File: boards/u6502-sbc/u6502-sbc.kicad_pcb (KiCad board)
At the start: 4 copper layers, 100 x 100 mm, 35 parts, among them J1 HDR_USR_PORT, J2 HDR_USR_PORT, J3 HDR_USR_PORT, J4 HDR_USR_PORT, J6 HDR_FTDI, J7 HDR_RS232, J8 KLDX-0202-BC, J9 HDR_CPU_BUS, SW1 SW_RST, SW2 SW_SPDT, U1 W65C02SxPL, U10 DS1813-5+, U2 AS7C256B-15PIN, U3 28C256, U4 W65C22SxPL, U5 W65C51NxP, U6 74HC00, U7 74HC21, U8 W65C22SxPL, U9 NCP1117IDT50T4G, X1 1MHz

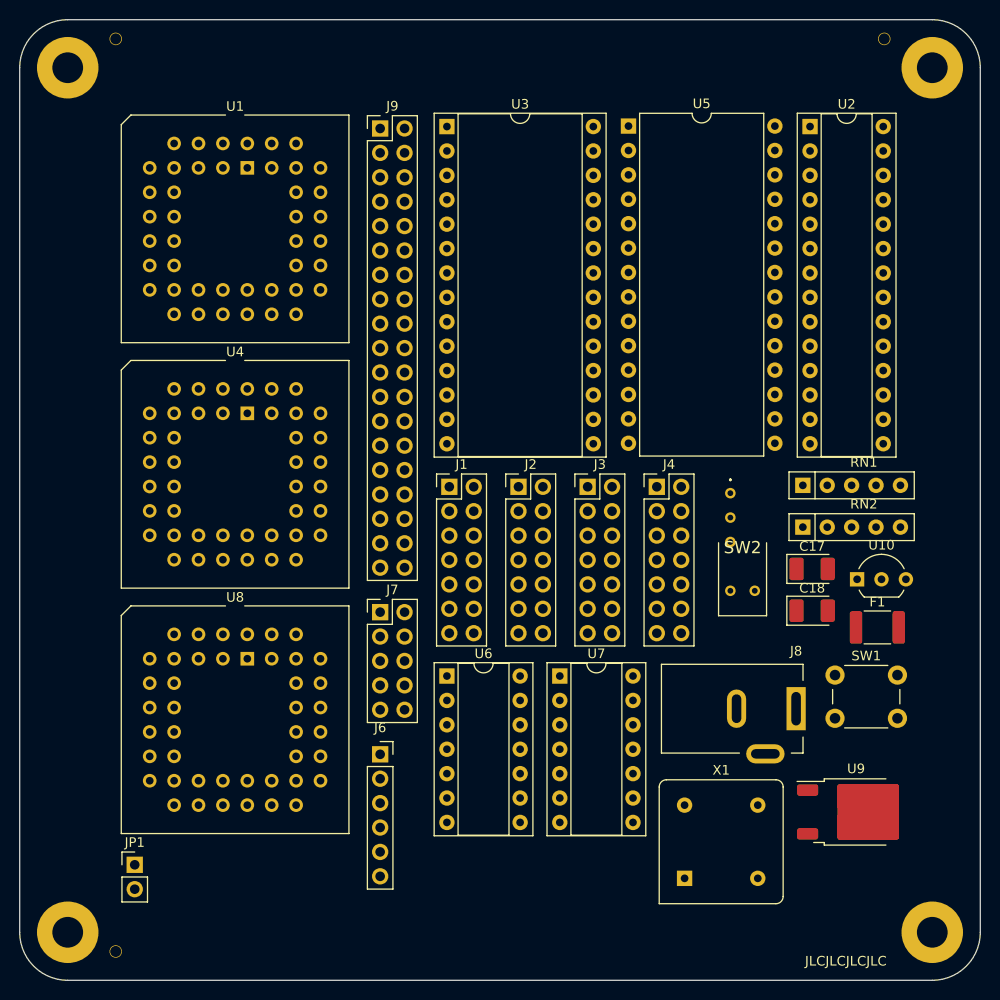
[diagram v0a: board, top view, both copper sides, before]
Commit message: Initial layout and routing wip
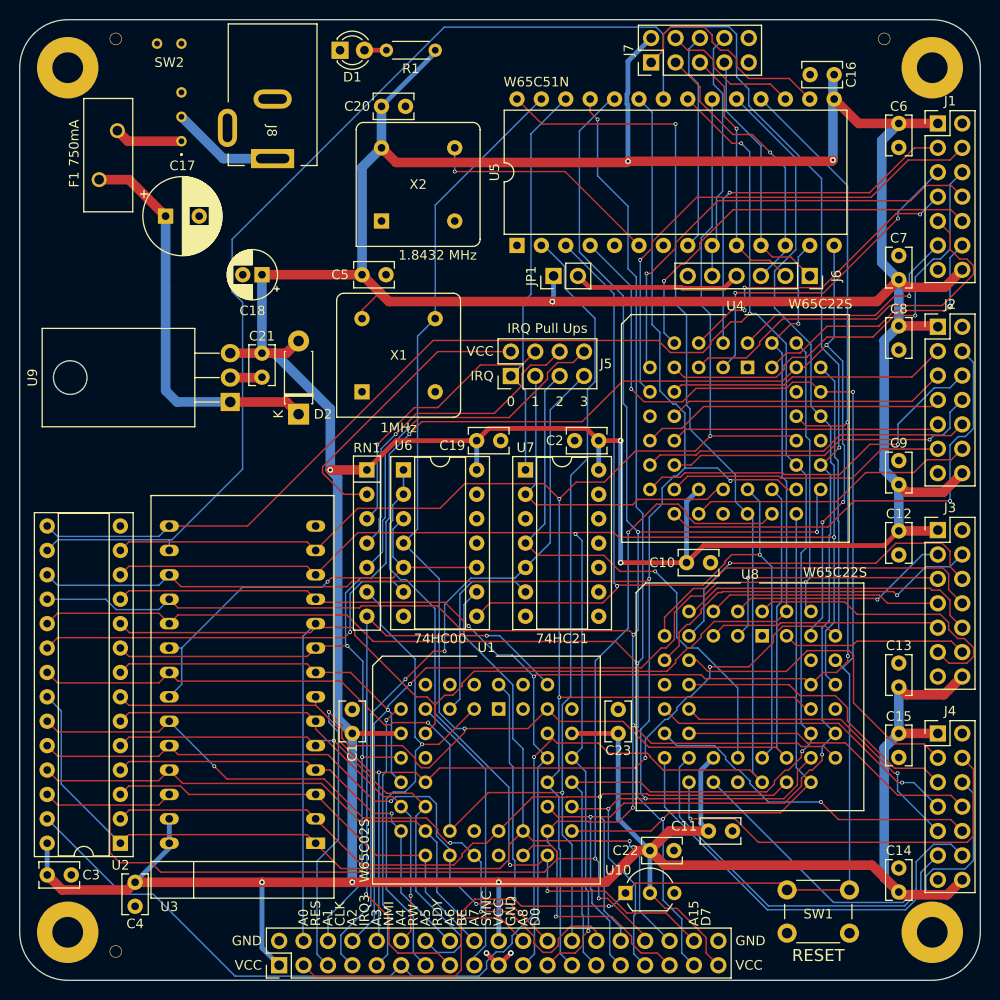
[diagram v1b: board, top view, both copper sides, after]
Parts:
- removed RN2: 3k3, Resistor_THT:R_Array_SIP5
- added C1: 100n, Capacitor_THT:C_Rect_L4.0mm_W2.5mm_P2.50mm, F.Cu at (134.6, 114.3)
- added C10: 100n, Capacitor_THT:C_Rect_L4.0mm_W2.5mm_P2.50mm, F.Cu at (169.4, 96.5)
- added C11: 100n, Capacitor_THT:C_Rect_L4.0mm_W2.5mm_P2.50mm, F.Cu at (171.7, 124.5)
- added C12: 100n, Capacitor_THT:C_Rect_L4.0mm_W2.5mm_P2.50mm, F.Cu at (191.5, 93.2)
- added C13: 100n, Capacitor_THT:C_Rect_L4.0mm_W2.5mm_P2.50mm, F.Cu at (191.5, 109.5)
- added C14: 100n, Capacitor_THT:C_Rect_L4.0mm_W2.5mm_P2.50mm, F.Cu at (191.5, 130.8)
- added C15: 100n, Capacitor_THT:C_Rect_L4.0mm_W2.5mm_P2.50mm, F.Cu at (191.5, 114.3)
- added C16: 100n, Capacitor_THT:C_Rect_L4.0mm_W2.5mm_P2.50mm, F.Cu at (184.8, 45.7)
- added C19: 100n, Capacitor_THT:C_Rect_L4.0mm_W2.5mm_P2.50mm, F.Cu at (147.6, 83.8)
- added C2: 100n, Capacitor_THT:C_Rect_L4.0mm_W2.5mm_P2.50mm, F.Cu at (160.3, 83.8)
- added C20: 100n, Capacitor_THT:C_Rect_L4.0mm_W2.5mm_P2.50mm, F.Cu at (140.2, 49.0)
- added C21: 100n, Capacitor_THT:C_Rect_L4.0mm_W2.5mm_P2.50mm, F.Cu at (125.2, 74.7)
- added C22: 100n, Capacitor_THT:C_Rect_L4.0mm_W2.5mm_P2.50mm, F.Cu at (165.6, 126.5)
- added C23: 100n, Capacitor_THT:C_Rect_L4.0mm_W2.5mm_P2.50mm, F.Cu at (162.3, 114.3)
- added C3: 100n, Capacitor_THT:C_Rect_L4.0mm_W2.5mm_P2.50mm, F.Cu at (102.9, 129.0)
- added C4: 100n, Capacitor_THT:C_Rect_L4.0mm_W2.5mm_P2.50mm, F.Cu at (112.0, 129.8)
- added C5: 100n, Capacitor_THT:C_Rect_L4.0mm_W2.5mm_P2.50mm, F.Cu at (135.6, 66.5)
- added C6: 100n, Capacitor_THT:C_Rect_L4.0mm_W2.5mm_P2.50mm, F.Cu at (191.5, 50.8)
- added C7: 100n, Capacitor_THT:C_Rect_L4.0mm_W2.5mm_P2.50mm, F.Cu at (191.5, 67.1)
- added C8: 100n, Capacitor_THT:C_Rect_L4.0mm_W2.5mm_P2.50mm, F.Cu at (191.5, 71.9)
- added C9: 100n, Capacitor_THT:C_Rect_L4.0mm_W2.5mm_P2.50mm, F.Cu at (191.5, 88.4)
- added D1: LED_PWR, LED_THT:LED_D3.0mm, F.Cu at (133.3, 43.2)
- added D2: 1N5819, Diode_THT:D_DO-41_SOD81_P7.62mm_Horizontal, F.Cu at (129.0, 81.1)
- added J5: HDR_IRQ, Connector_PinHeader_2.54mm:PinHeader_2x04_P2.54mm_Vertical, F.Cu at (151.1, 77.1)
- added R1: 1k, Resistor_THT:R_Axial_DIN0204_L3.6mm_D1.6mm_P5.08mm_Horizontal, F.Cu at (143.3, 43.2)
- added X2: 1.8432 MHz, Oscillator:Oscillator_DIP-8, F.Cu at (137.7, 61.0)
- C17: footprint Capacitor_Tantalum_SMD:CP_EIA-3528-21_Kemet-B_Pad1.50x2.35mm_HandSolder -> Capacitor_THT:CP_Radial_D8.0mm_P3.50mm
- C18: value 10u -> 4u7; footprint Capacitor_Tantalum_SMD:CP_EIA-3528-21_Kemet-B_Pad1.50x2.35mm_HandSolder -> Capacitor_THT:CP_Radial_D5.0mm_P2.00mm
- F1: footprint Fuse:Fuse_1812_4532Metric_Pad1.30x3.40mm_HandSolder -> Fuse:Fuse_BelFuse_0ZRE0075FF_L11.5mm_W4.8mm
- RN1: footprint Resistor_THT:R_Array_SIP5 -> Resistor_THT:R_Array_SIP7
- SYM1: moved to B.Cu
- U3: footprint Package_DIP:DIP-28_W15.24mm_Socket -> Mouser:Aries 28-526-10
- U9: value NCP1117IDT50T4G -> L7805CV; footprint Package_TO_SOT_SMD:TO-252-2 -> Package_TO_SOT_THT:TO-220-3_Horizontal_TabDown
- moved U2 103.5 mm to (110.5, 125.7), turned to 180 degrees
- moved F1 94.5 mm to (110.2, 51.6), turned to -90 degrees
- moved locked 87.7 mm to (127.0, 138.4), turned to 90 degrees
- moved J8 79.1 mm to (126.3, 54.5), turned to -90 degrees
- moved U9 77.9 mm to (121.9, 79.8), turned to 90 degrees
- moved C17 76.7 mm to (115.2, 60.5)
- moved JP1 75.2 mm to (155.6, 66.7), turned to 90 degrees
- moved SW2 67.9 mm to (116.8, 52.6), turned to 180 degrees
- moved C18 67.1 mm to (125.2, 66.5), turned to 180 degrees
- moved J6 66.9 mm to (182.2, 66.7), turned to -90 degrees
- moved J7 63.8 mm to (165.7, 44.5), turned to 90 degrees
- moved J1 63.4 mm to (195.6, 50.8)
- moved U1 62.1 mm to (149.9, 111.8)
- moved U3 61.9 mm to (123.2, 109.2), turned to 180 degrees
- moved X1 60.8 mm to (135.6, 78.7)
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- renumbered J9 to locked
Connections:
- net Net-(J6-Pin_4) renamed /ftdi_vcc
- J1 pad 11: /PA5 -> /CA1
- J1 pad 12: /PA6 -> /CA2
- J1 pad 13: /PA7 -> GND
- J1 pad 14: GND -> VCC
- J1 pad 2: /PA0 -> GND
- J1 pad 3: /PA1 -> /PA0
- J1 pad 4: /PA2 -> /PA7
- J1 pad 5: /PA3 -> /PA1
- J1 pad 6: /CA1 -> /PA6
- J1 pad 7: GND -> /PA2
- J1 pad 8: VCC -> /PA5
- J1 pad 9: /CA2 -> /PA3
- J2 pad 11: /PB5 -> /CB1
- J2 pad 12: /PB6 -> /CB2
- J2 pad 13: /PB7 -> GND
- J2 pad 14: GND -> VCC
- J2 pad 2: /PB0 -> GND
- J2 pad 3: /PB1 -> /PB0
- J2 pad 4: /PB2 -> /PB7
- J2 pad 5: /PB3 -> /PB1
- J2 pad 6: /CB1 -> /PB6
- J2 pad 7: GND -> /PB2
- J2 pad 8: VCC -> /PB5
- J2 pad 9: /CB2 -> /PB3
- J3 pad 11: /PC5 -> /CC1
- J3 pad 12: /PC6 -> /CC2
- J3 pad 13: /PC7 -> GND
- J3 pad 14: GND -> VCC
- J3 pad 2: /PC0 -> GND
- J3 pad 3: /PC1 -> /PC0
- J3 pad 4: /PC2 -> /PC7
- J3 pad 5: /PC3 -> /PC1
- J3 pad 6: /CC1 -> /PC6
- J3 pad 7: GND -> /PC2
- J3 pad 8: VCC -> /PC5
- J3 pad 9: /CC2 -> /PC3
- J4 pad 11: /PD5 -> /CD1
- J4 pad 12: /PD6 -> /CD2
- J4 pad 13: /PD7 -> GND
- J4 pad 14: GND -> VCC
- J4 pad 2: /PD0 -> GND
- J4 pad 3: /PD1 -> /PD0
- J4 pad 4: /PD2 -> /PD7
- J4 pad 5: /PD3 -> /PD1
- J4 pad 6: /CD1 -> /PD6
- J4 pad 7: GND -> /PD2
- J4 pad 8: VCC -> /PD5
- J4 pad 9: /CD2 -> /PD3
- SW1 pad 1: /~{RST} -> /~{RES}
- U1 pad 3: unconnected-(U1-RDY-Pad3) -> /RDY
- U1 pad 40: unconnected-(U1-BE-Pad40) -> /BE
- U1 pad 8: unconnected-(U1-SYNC-Pad8) -> /SYNC
- U10 pad 1: /~{RST} -> /~{RES}
- U5 pad 6: unconnected-(U5-XTAL1-Pad6) -> /ACIA_XTAL
- U8 pad 25: unconnected-(U8-~{CS2}-Pad25) -> /IO_~{CS}
- U9 pad 1: GND -> VDC
- U9 pad 2: VCC -> GND
- U9 pad 3: VDC -> VCC
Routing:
- net VCC: track 0.00 -> 634.7 mm, vias 0 -> 9
- net /D4: track 0.00 -> 250.2 mm, vias 0 -> 3
- net /D6: track 0.00 -> 221.3 mm, vias 0 -> 6
- net /D7: track 0.00 -> 215.8 mm, vias 0 -> 3
- net /D3: track 0.00 -> 206.1 mm, vias 0 -> 3
- net /D5: track 0.00 -> 200.4 mm, vias 0 -> 4
- net /R~{W}: track 0.00 -> 195.4 mm, vias 0 -> 2
- net /D1: track 0.00 -> 194.0 mm, vias 0 -> 3
- net /D2: track 0.00 -> 190.3 mm, vias 0 -> 3
- net /CLK: track 0.00 -> 187.8 mm, vias 0 -> 2
- net /~{RES}: track 0.00 -> 184.4 mm, vias 0 -> 4
- net /D0: track 0.00 -> 181.2 mm, vias 0 -> 4
- net /A1: track 0.00 -> 177.4 mm, vias 0 -> 6
- net /A0: track 0.00 -> 156.3 mm, vias 0 -> 1
- net /A10: track 0.00 -> 145.2 mm, vias 0 -> 2
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- added copper zone on In1.Cu, net GND
- added copper zone on In2.Cu, net GND
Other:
- board text added: "0"
- board text added: "1"
- board text added: "2"
- board text added: "3"
- board text added: "A0"
- board text added: "A1"
- board text added: "A15"
- board text added: "A2"
- board text added: "A3"
- board text added: "A4"
- board text added: "A5"
- board text added: "A6"
- board text added: "A7"
- board text added: "A8"
- board text added: "BE"
- board text added: "CLK"
- board text added: "D0"
- board text added: "D7"
- board text added: "GND"
- board text added: "IRQ"
- board text added: "IRQ Pull Ups"
- board text added: "IRQ3"
- board text added: "NMI"
- board text added: "RDY"
- board text added: "RES"
- board text added: "RESET"
- board text added: "RW"
- board text added: "SYNC"
- board text added: "VCC"
- board text added: "W65C02S"
- board text added: "W65C22S"
- board text added: "W65C51N"
